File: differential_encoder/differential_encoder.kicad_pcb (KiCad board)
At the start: 2 copper layers, 92.7 x 40.4 mm, 43 parts, among them J101 Conn_01x12, J102 RJ45_LED_Shielded, J103 RJ45_LED_Shielded, Q101 Q_NMOS_GSD, Q102 Q_NMOS_GSD, Q103 Q_NMOS_GSD, Q104 Q_NMOS_GSD, Q105 Q_NMOS_GSD, Q106 Q_NMOS_GSD, U101 MAX489E, U102 MAX489E, U103 MAX489E, U104 MAX489E, U105 MAX489E, U106 MAX489E

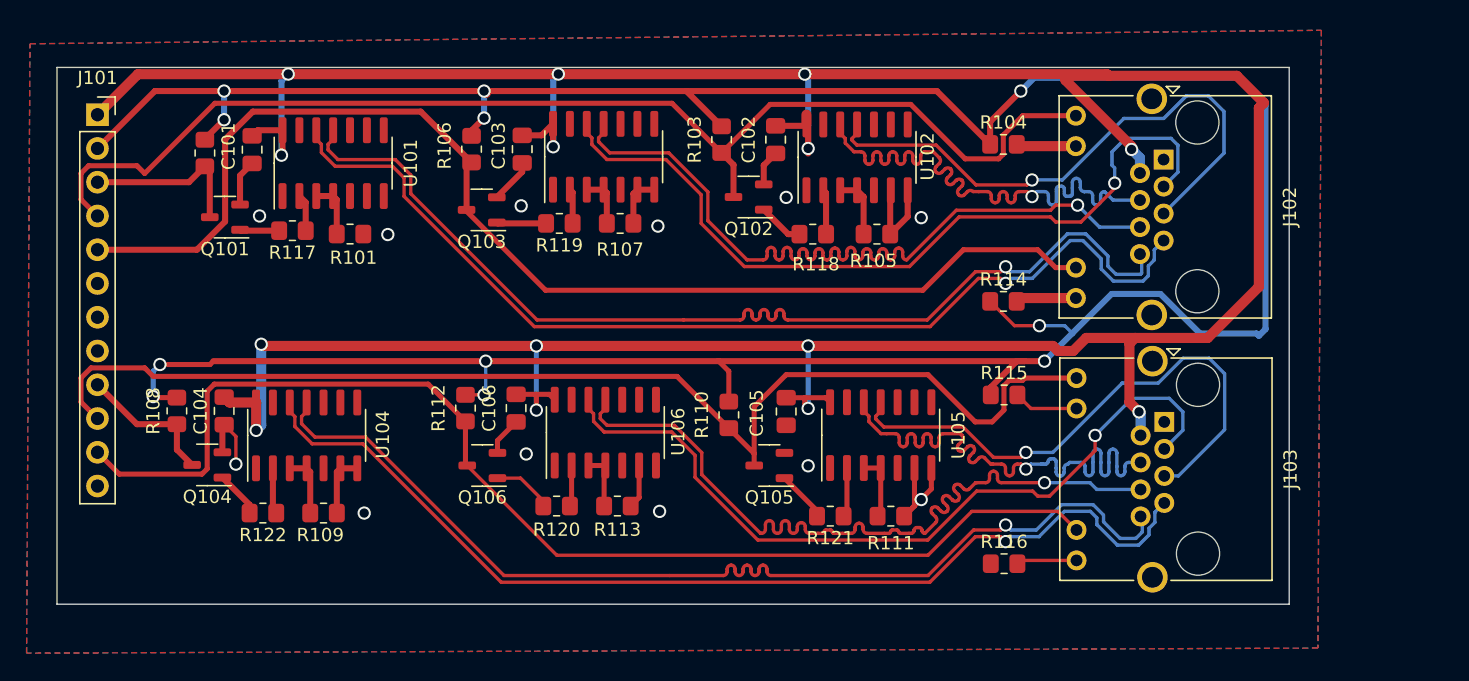
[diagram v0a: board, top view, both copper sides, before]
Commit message: final version odrive
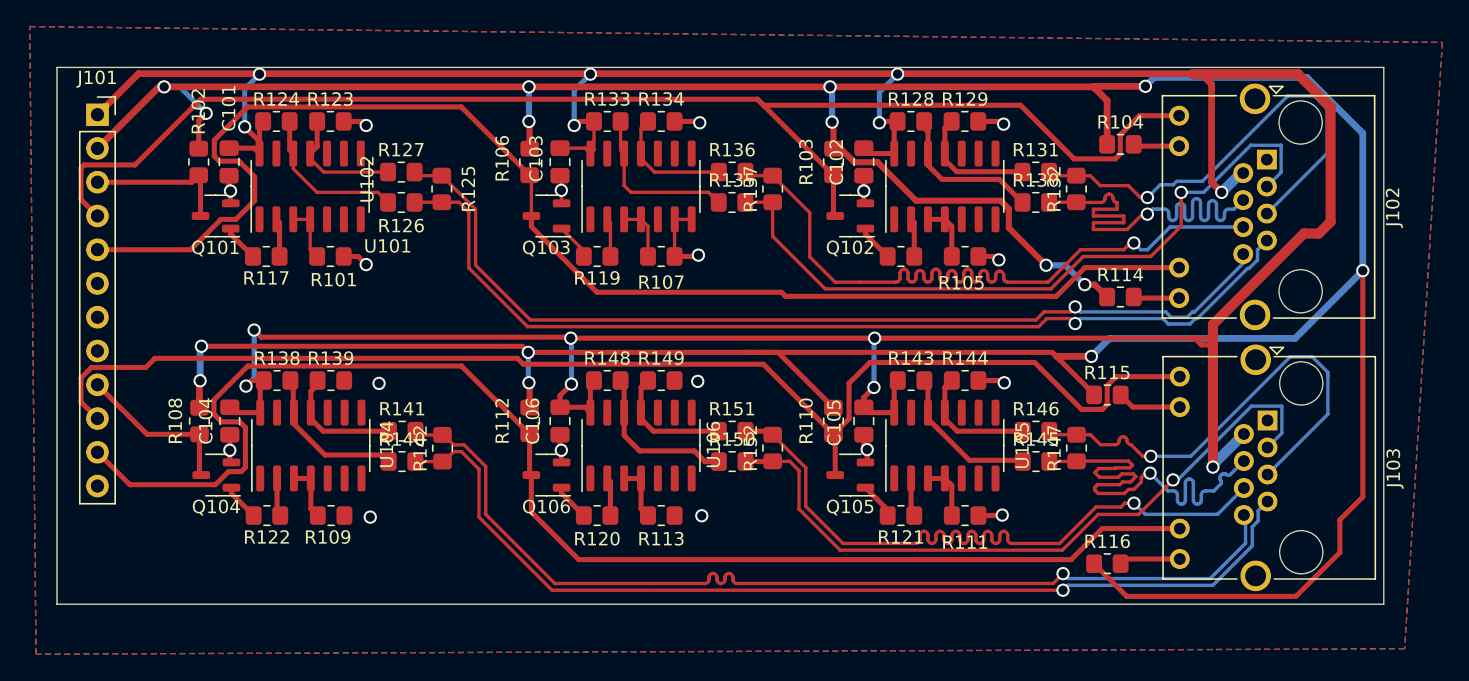
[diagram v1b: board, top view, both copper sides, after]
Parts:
- added R123: 10k, Resistor_SMD:R_0805_2012Metric_Pad1.20x1.40mm_HandSolder, F.Cu at (96.3, 71.6)
- added R124: 10k, Resistor_SMD:R_0805_2012Metric_Pad1.20x1.40mm_HandSolder, F.Cu at (92.2, 71.6)
- added R125: 10k, Resistor_SMD:R_0805_2012Metric_Pad1.20x1.40mm_HandSolder, F.Cu at (104.6, 76.7)
- added R126: 10k, Resistor_SMD:R_0805_2012Metric_Pad1.20x1.40mm_HandSolder, F.Cu at (101.6, 77.7)
- added R127: 10k, Resistor_SMD:R_0805_2012Metric_Pad1.20x1.40mm_HandSolder, F.Cu at (101.6, 75.4)
- added R128: 10k, Resistor_SMD:R_0805_2012Metric_Pad1.20x1.40mm_HandSolder, F.Cu at (139.9, 71.6)
- added R129: 10k, Resistor_SMD:R_0805_2012Metric_Pad1.20x1.40mm_HandSolder, F.Cu at (144.0, 71.6)
- added R130: 10k, Resistor_SMD:R_0805_2012Metric_Pad1.20x1.40mm_HandSolder, F.Cu at (149.3, 77.7)
- added R131: 10k, Resistor_SMD:R_0805_2012Metric_Pad1.20x1.40mm_HandSolder, F.Cu at (149.3, 75.4)
- added R132: 10k, Resistor_SMD:R_0805_2012Metric_Pad1.20x1.40mm_HandSolder, F.Cu at (152.4, 76.7)
- added R133: 10k, Resistor_SMD:R_0805_2012Metric_Pad1.20x1.40mm_HandSolder, F.Cu at (117.1, 71.6)
- added R134: 10k, Resistor_SMD:R_0805_2012Metric_Pad1.20x1.40mm_HandSolder, F.Cu at (121.2, 71.6)
- added R135: 10k, Resistor_SMD:R_0805_2012Metric_Pad1.20x1.40mm_HandSolder, F.Cu at (126.5, 77.7)
- added R136: 10k, Resistor_SMD:R_0805_2012Metric_Pad1.20x1.40mm_HandSolder, F.Cu at (126.5, 75.4)
- added R137: 10k, Resistor_SMD:R_0805_2012Metric_Pad1.20x1.40mm_HandSolder, F.Cu at (129.5, 76.7)
- added R138: 10k, Resistor_SMD:R_0805_2012Metric_Pad1.20x1.40mm_HandSolder, F.Cu at (92.3, 91.1)
- added R139: 10k, Resistor_SMD:R_0805_2012Metric_Pad1.20x1.40mm_HandSolder, F.Cu at (96.3, 91.1)
- added R140: 10k, Resistor_SMD:R_0805_2012Metric_Pad1.20x1.40mm_HandSolder, F.Cu at (101.7, 97.2)
- added R141: 10k, Resistor_SMD:R_0805_2012Metric_Pad1.20x1.40mm_HandSolder, F.Cu at (101.7, 94.9)
- added R142: 10k, Resistor_SMD:R_0805_2012Metric_Pad1.20x1.40mm_HandSolder, F.Cu at (104.7, 96.2)
- added R143: 10k, Resistor_SMD:R_0805_2012Metric_Pad1.20x1.40mm_HandSolder, F.Cu at (140.0, 91.1)
- added R144: 10k, Resistor_SMD:R_0805_2012Metric_Pad1.20x1.40mm_HandSolder, F.Cu at (144.0, 91.1)
- added R145: 10k, Resistor_SMD:R_0805_2012Metric_Pad1.20x1.40mm_HandSolder, F.Cu at (149.4, 97.2)
- added R146: 10k, Resistor_SMD:R_0805_2012Metric_Pad1.20x1.40mm_HandSolder, F.Cu at (149.4, 94.9)
- added R147: 10k, Resistor_SMD:R_0805_2012Metric_Pad1.20x1.40mm_HandSolder, F.Cu at (152.4, 96.2)
- added R148: 10k, Resistor_SMD:R_0805_2012Metric_Pad1.20x1.40mm_HandSolder, F.Cu at (117.1, 91.1)
- added R149: 10k, Resistor_SMD:R_0805_2012Metric_Pad1.20x1.40mm_HandSolder, F.Cu at (121.2, 91.1)
- added R150: 10k, Resistor_SMD:R_0805_2012Metric_Pad1.20x1.40mm_HandSolder, F.Cu at (126.5, 97.2)
- added R151: 10k, Resistor_SMD:R_0805_2012Metric_Pad1.20x1.40mm_HandSolder, F.Cu at (126.5, 94.9)
- added R152: 10k, Resistor_SMD:R_0805_2012Metric_Pad1.20x1.40mm_HandSolder, F.Cu at (129.5, 96.2)
- moved R114 8.81 mm to (155.7, 84.8)
- moved R104 8.80 mm to (155.7, 73.4)
- moved R103 8.58 mm to (134.1, 74.7)
- moved R110 7.89 mm to (134.1, 94.2)
- moved Q102 7.78 mm to (135.4, 78.7)
- moved J103 7.77 mm to (166.8, 94.1)
- moved J102 7.77 mm to (166.7, 74.5)
- moved R115 7.77 mm to (154.7, 92.2)
- moved R116 7.77 mm to (154.7, 104.9)
- moved U102 6.96 mm to (142.5, 76.5)
- moved C102 6.85 mm to (136.4, 74.7)
- moved R105 6.85 mm to (144.0, 81.8)
- moved R118 6.85 mm to (139.2, 81.8)
- moved Q105 6.14 mm to (135.4, 98.2)
- moved C105 5.89 mm to (136.4, 94.2)
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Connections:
- U101 pad 11: a1- -> Net-(U101-B)
- U101 pad 12: a1+ -> Net-(U101-A)
- U102 pad 11: b1- -> Net-(U102-B)
- U102 pad 12: b1+ -> Net-(U102-A)
- U103 pad 11: i1- -> Net-(U103-B)
- U103 pad 12: i1+ -> Net-(U103-A)
- U104 pad 11: a0- -> Net-(U104-B)
- U104 pad 12: a0+ -> Net-(U104-A)
- U105 pad 11: b0- -> Net-(U105-B)
- U105 pad 12: b0+ -> Net-(U105-A)
- U106 pad 11: i0- -> Net-(U106-B)
- U106 pad 12: i0+ -> Net-(U106-A)
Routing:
- net +3V3: track 233.9 -> 312.0 mm, vias 11 -> 15
- net +5V: track 262.9 -> 282.4 mm
- net I0: track 89.7 -> 103.6 mm
- net GND: track 45.5 -> 32.0 mm, vias 12 -> 18
- net Net-(U103-A): track 0.00 -> 12.6 mm
- net B1: track 91.9 -> 104.1 mm
- net Net-(U106-A): track 0.00 -> 12.2 mm
- net Net-(U101-A): track 0.00 -> 11.8 mm
- net Net-(U102-A): track 0.00 -> 11.7 mm
- net Net-(U104-A): track 0.00 -> 11.7 mm
- net Net-(U105-A): track 0.00 -> 11.5 mm
- net I1: track 91.6 -> 102.6 mm
- net Net-(U104-B): track 0.00 -> 9.35 mm
- net Net-(U106-B): track 0.00 -> 9.34 mm
- net Net-(U105-B): track 0.00 -> 9.34 mm
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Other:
- board size 92.7 x 40.4 mm -> 99.8 x 40.4 mm
